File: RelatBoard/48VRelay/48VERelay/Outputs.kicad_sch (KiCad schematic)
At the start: 16 parts, among them J10 Screw_Terminal_01x03, J11 Screw_Terminal_01x03, J12 Screw_Terminal_01x03, J13 Screw_Terminal_01x03, J14 Screw_Terminal_01x03, K10 G2RL-1-E, K11 G2RL-1-E, K12 G2RL-1-E, K13 G2RL-1-E, K14 G2RL-1-E, U1 ULN2803A

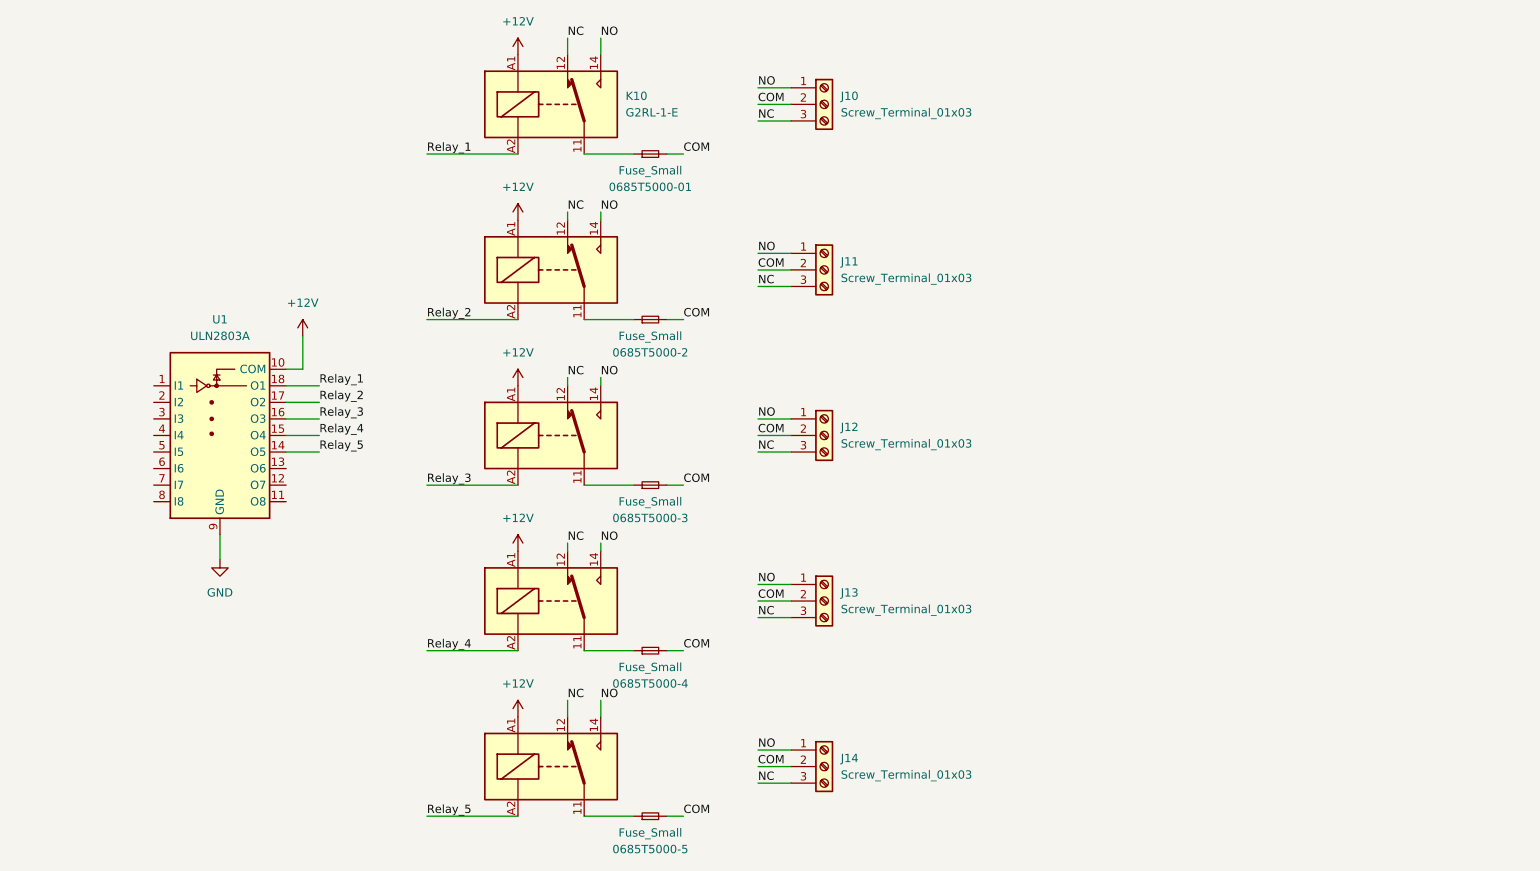
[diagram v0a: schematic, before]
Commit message: sys_update
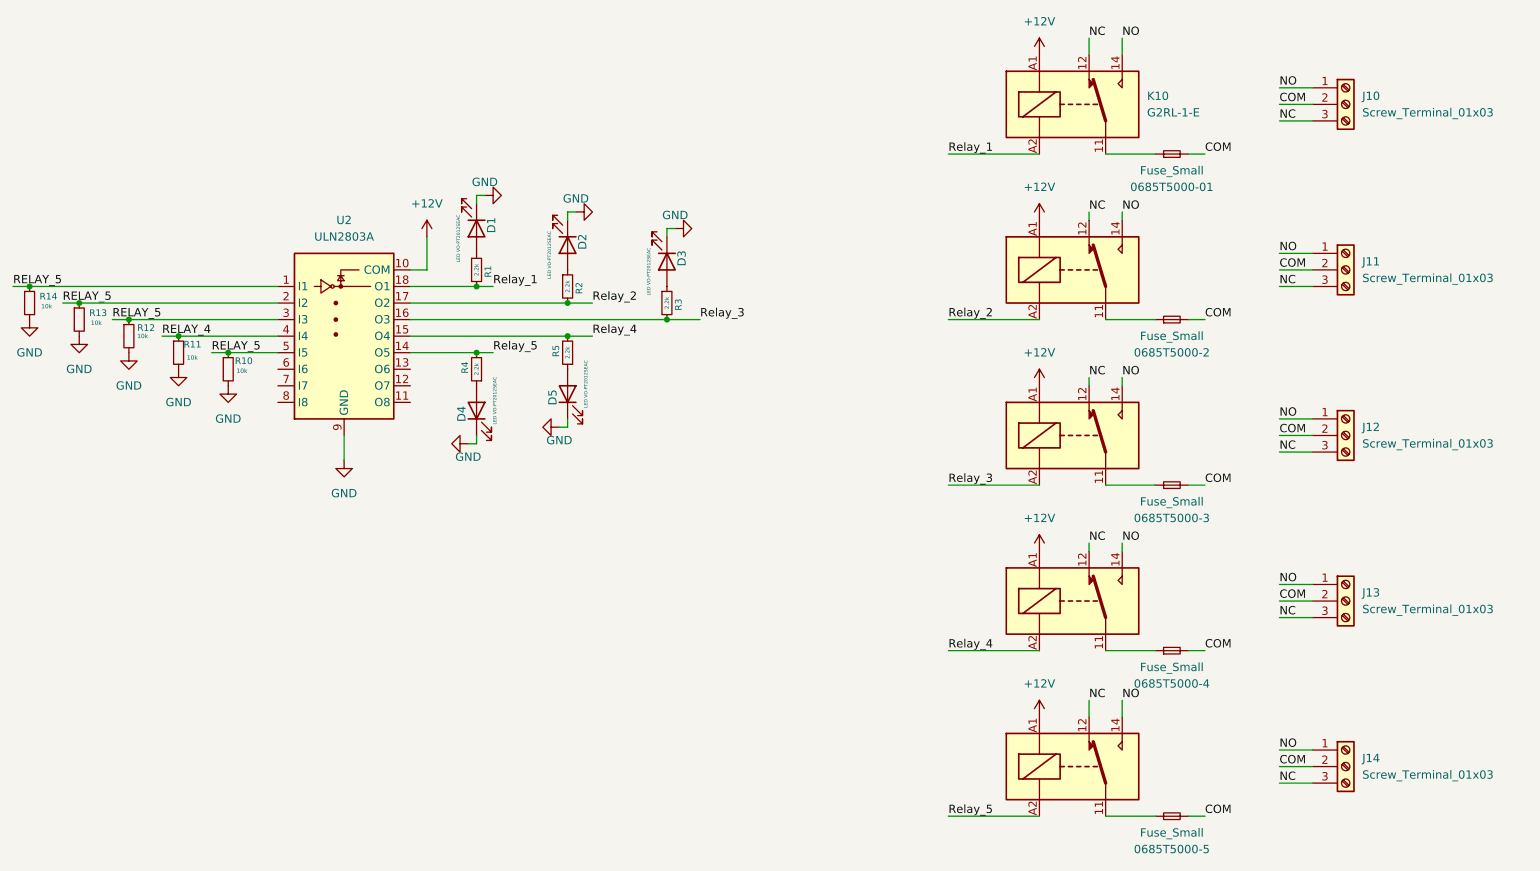
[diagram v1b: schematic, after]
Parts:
- added D1, D2, D3, D4, D5: LED VO-PT2012SEAC, symbol Device:LED
- added R1, R2, R3, R4, R5: 2.2k, symbol Device:R_Small
- added R10, R11, R12, R13, R14: 10k, symbol Device:R_Small
- renumbered U1 to U2
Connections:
- net GND: now also D1.1 (K), D2.1 (K), D3.1 (K), D4.1 (K), D5.1 (K), R10.2, R11.2, R12.2, R13.2, R14.2
- net Relay_1: now also R1.2
- net Relay_2: now also R2.2
- net Relay_3: now also R3.2
- net Relay_4: now also R5.2
- net Relay_5: now also R4.2
- net RELAY_5: now reaches U2.1 (I1)
- net RELAY_5: now also U2.2 (I2), U2.3 (I3), U2.5 (I5), R10.1, R12.1, R13.1, R14.1
- net RELAY_4: now reaches U2.4 (I4)
- net RELAY_4: now also R11.1
- new net: D2.2 (A), R2.1
- new net: D5.2 (A), R5.1
- new net: D4.2 (A), R4.1
- new net: D3.2 (A), R3.1
- new net: D1.2 (A), R1.1
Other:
- moved on the sheet: 0685T5000-01, 0685T5000-2, 0685T5000-3, 0685T5000-4, 0685T5000-5, J10, J11, J12, J13, J14, K10, U2

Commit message: begin pcb design
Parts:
- 0685T5000-2, 0685T5000-3, 0685T5000-4, 0685T5000-5: footprint (none) -> Fuse:Fuse_0603_1608Metric
- D1, D2, D3, D4, D5: footprint (none) -> LED_SMD:LED_0201_0603Metric
- R1, R10, R11, R12, R13, R14, R2, R3, R4, R5: footprint (none) -> Resistor_SMD:R_0603_1608Metric
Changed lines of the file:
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@@
 		(unit 1)
 		(body_style 1)
-		(exclude_from_sim no)
+		(exclude_from_sim yes)
 		(in_bom yes)
 		(on_board yes)
@@
 			)
 		)
-		(property "Footprint" ""
+		(property "Footprint" "Resistor_SMD:R_0603_1608Metric"
 			(at 129.54 66.04 0)
 			(hide yes)
@@
 			)
 		)
-		(property "Footprint" ""
+		(property "Footprint" "Fuse:Fuse_0603_1608Metric"
 			(at 222.25 121.92 0)
 			(hide yes)
@@
 			)
 		)
-		(property "Footprint" ""
+		(property "Footprint" "Resistor_SMD:R_0603_1608Metric"
 			(at 129.54 76.2 0)
 			(hide yes)
@@
 		(unit 1)
 		(body_style 1)
-		(exclude_from_sim no)
+		(exclude_from_sim yes)
 		(in_bom yes)
 		(on_board yes)
@@
 			)
 		)
-		(property "Footprint" ""
+		(property "Footprint" "Fuse:Fuse_0603_1608Metric"
 			(at 222.25 96.52 0)
 			(hide yes)
@@
 			)
 		)
-		(property "Footprint" ""
+		(property "Footprint" "Resistor_SMD:R_0603_1608Metric"
 			(at 77.47 78.74 0)
 			(hide yes)
@@
 			)
 		)
-		(property "Footprint" ""
+		(property "Footprint" "Fuse:Fuse_0603_1608Metric"
 			(at 222.25 71.12 0)
 			(hide yes)
@@
 			)
 		)
-		(property "Footprint" ""
+		(property "Footprint" "Fuse:Fuse_0603_1608Metric"
 			(at 222.25 147.32 0)
 			(hide yes)
@@
 			)
 		)
-		(property "Footprint" ""
+		(property "Footprint" "Resistor_SMD:R_0603_1608Metric"
 			(at 54.61 71.12 0)
 			(hide yes)
@@
 			)
 		)
-		(property "Footprint" ""
+		(property "Footprint" "LED_SMD:LED_0201_0603Metric"
 			(at 115.57 85.09 0)
 			(hide yes)
@@
 		(unit 1)
 		(body_style 1)
-		(exclude_from_sim no)
+		(exclude_from_sim yes)
 		(in_bom yes)
 		(on_board yes)
@@
 			)
 		)
-		(property "Footprint" ""
+		(property "Footprint" "Resistor_SMD:R_0603_1608Metric"
 			(at 144.78 68.58 0)
 			(hide yes)
@@
 			)
 		)
-		(property "Footprint" ""
+		(property "Footprint" "LED_SMD:LED_0201_0603Metric"
 			(at 129.54 59.69 0)
 			(hide yes)
@@
 			)
 		)
-		(property "Footprint" ""
+		(property "Footprint" "LED_SMD:LED_0201_0603Metric"
 			(at 129.54 82.55 0)
 			(hide yes)
@@
 		(instances
 			(project "48VERelay"
-				(path "/2d740e7a-a48e-41b8-b74e-ca0ab277f7d9"
-					(reference "#PWR06")
-					(unit 1)
-				)
 				(path "/2d740e7a-a48e-41b8-b74e-ca0ab277f7d9/9acca724-bbf8-479c-b765-a30537109626"
 					(reference "#PWR06")
@@
 			)
 		)
-		(property "Footprint" ""
+		(property "Footprint" "Resistor_SMD:R_0603_1608Metric"
 			(at 69.85 76.2 0)
 			(hide yes)
@@
 		(unit 1)
 		(body_style 1)
-		(exclude_from_sim no)
+		(exclude_from_sim yes)
 		(in_bom yes)
 		(on_board yes)
@@
 		(unit 1)
 		(body_style 1)
-		(exclude_from_sim no)
+		(exclude_from_sim yes)
 		(in_bom yes)
 		(on_board yes)
@@
 		(instances
 			(project "48VERelay"
-				(path "/2d740e7a-a48e-41b8-b74e-ca0ab277f7d9"
-					(reference "0685T5000-01")
-					(unit 1)
-				)
 				(path "/2d740e7a-a48e-41b8-b74e-ca0ab277f7d9/9acca724-bbf8-479c-b765-a30537109626"
 					(reference "0685T5000-01")
@@
 			)
 		)
-		(property "Footprint" ""
+		(property "Footprint" "Resistor_SMD:R_0603_1608Metric"
 			(at 115.57 63.5 0)
 			(hide yes)
@@
 			)
 		)
-		(property "Footprint" ""
+		(property "Footprint" "Resistor_SMD:R_0603_1608Metric"
 			(at 115.57 78.74 0)
 			(hide yes)
@@
 		(instances
 			(project "48VERelay"
-				(path "/2d740e7a-a48e-41b8-b74e-ca0ab277f7d9"
-					(reference "#PWR01")
-					(unit 1)
-				)
 				(path "/2d740e7a-a48e-41b8-b74e-ca0ab277f7d9/9acca724-bbf8-479c-b765-a30537109626"
 					(reference "#PWR01")
@@
 			)
 		)
-		(property "Footprint" ""
+		(property "Footprint" "Resistor_SMD:R_0603_1608Metric"
 			(at 46.99 68.58 0)
 			(hide yes)
@@
 			)
 		)
-		(property "Footprint" ""
+		(property "Footprint" "Resistor_SMD:R_0603_1608Metric"
 			(at 62.23 73.66 0)
 			(hide yes)
@@
 			)
 		)
-		(property "Footprint" ""
+		(property "Footprint" "LED_SMD:LED_0201_0603Metric"
 			(at 144.78 62.23 0)
 			(hide yes)
@@
 			)
 		)
-		(property "Footprint" ""
+		(property "Footprint" "LED_SMD:LED_0201_0603Metric"
 			(at 115.57 57.15 0)
 			(hide yes)
@@
 		(instances
 			(project "48VERelay"
-				(path "/2d740e7a-a48e-41b8-b74e-ca0ab277f7d9"
-					(reference "U1")
-					(unit 1)
-				)
 				(path "/2d740e7a-a48e-41b8-b74e-ca0ab277f7d9/9acca724-bbf8-479c-b765-a30537109626"
 					(reference "U2")
